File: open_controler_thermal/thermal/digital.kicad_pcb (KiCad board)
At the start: 2 copper layers, 56 x 85 mm, 6 parts, among them J1 d_o_01x10, J2 d_i_01x10, J3 Conn_02x20_Odd_Even, J4 Conn_01x02

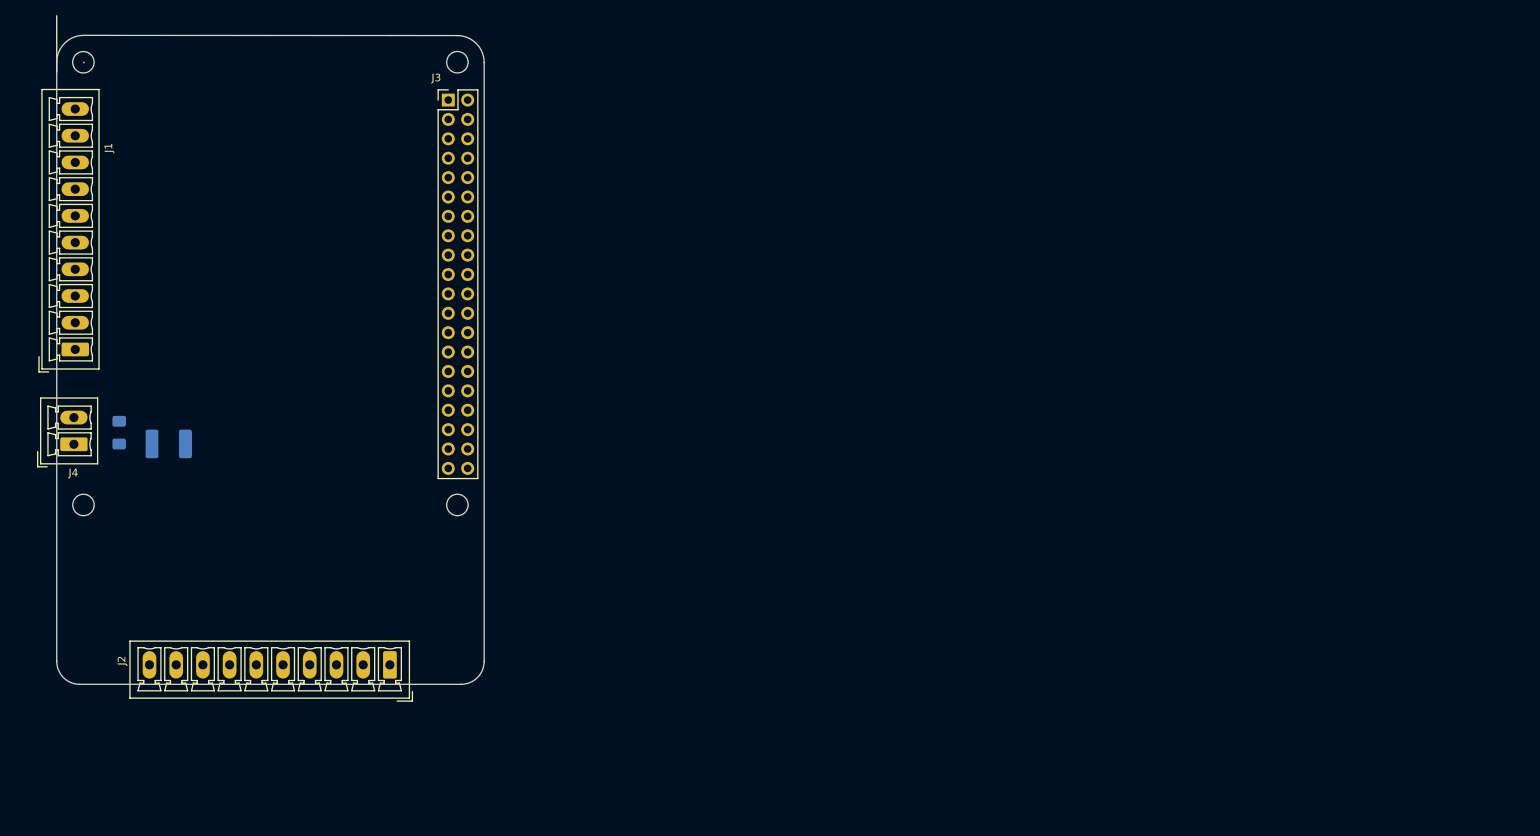
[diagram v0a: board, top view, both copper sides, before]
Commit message: trabajando en openControllerDigital
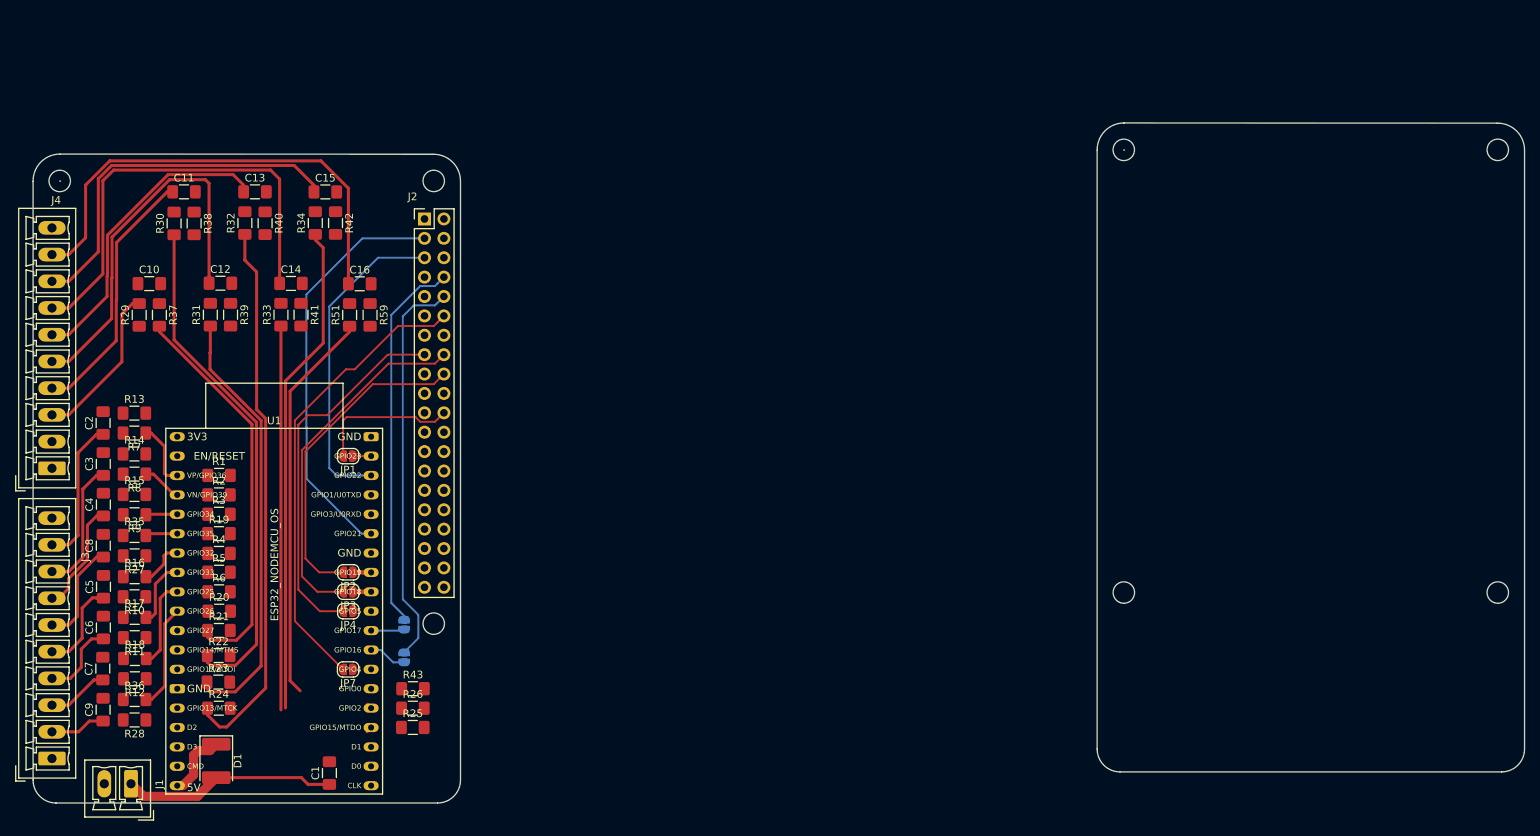
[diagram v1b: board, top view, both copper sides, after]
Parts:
- removed the J1 at (75.7, 82.8)
- added C1: 10nF, Capacitor_SMD:C_1206_3216Metric_Pad1.42x1.75mm_HandSolder, F.Cu at (109.0, 138.3)
- added C10: 10nF, Capacitor_SMD:C_1206_3216Metric_Pad1.42x1.75mm_HandSolder, F.Cu at (85.4, 74.2)
- added C11: 10nF, Capacitor_SMD:C_1206_3216Metric_Pad1.42x1.75mm_HandSolder, F.Cu at (90.0, 62.2)
- added C12: 10nF, Capacitor_SMD:C_1206_3216Metric_Pad1.42x1.75mm_HandSolder, F.Cu at (94.7, 74.1)
- added C13: 10nF, Capacitor_SMD:C_1206_3216Metric_Pad1.42x1.75mm_HandSolder, F.Cu at (99.2, 62.2)
- added C14: 10nF, Capacitor_SMD:C_1206_3216Metric_Pad1.42x1.75mm_HandSolder, F.Cu at (104.0, 74.2)
- added C15: 10nF, Capacitor_SMD:C_1206_3216Metric_Pad1.42x1.75mm_HandSolder, F.Cu at (108.5, 62.2)
- added C16: 10nF, Capacitor_SMD:C_1206_3216Metric_Pad1.42x1.75mm_HandSolder, F.Cu at (113.0, 74.2)
- added C2: 10nF, Capacitor_SMD:C_1206_3216Metric_Pad1.42x1.75mm_HandSolder, F.Cu at (79.3, 92.5)
- added C3: 10nF, Capacitor_SMD:C_1206_3216Metric_Pad1.42x1.75mm_HandSolder, F.Cu at (79.4, 97.8)
- added C4: 10nF, Capacitor_SMD:C_1206_3216Metric_Pad1.42x1.75mm_HandSolder, F.Cu at (79.4, 103.2)
- added C5: 10nF, Capacitor_SMD:C_1206_3216Metric_Pad1.42x1.75mm_HandSolder, F.Cu at (79.4, 113.9)
- added C6: 10nF, Capacitor_SMD:C_1206_3216Metric_Pad1.42x1.75mm_HandSolder, F.Cu at (79.4, 119.3)
- added C8: 10nF, Capacitor_SMD:C_1206_3216Metric_Pad1.42x1.75mm_HandSolder, F.Cu at (79.4, 108.5)
- added C9: 10nF, Capacitor_SMD:C_1206_3216Metric_Pad1.42x1.75mm_HandSolder, F.Cu at (79.3, 130.0)
- added J4: e_i_01x10, Connector_Phoenix_MC:PhoenixContact_MCV_1,5_10-G-3.5_1x10_P3.50mm_Vertical, F.Cu at (72.7, 98.4)
- added JP1: 23, Jumper:SolderJumper-2_P1.3mm_Open_RoundedPad1.0x1.5mm, F.Cu at (111.5, 96.8)
- added JP2: 19, Jumper:SolderJumper-2_P1.3mm_Open_RoundedPad1.0x1.5mm, F.Cu at (111.5, 112.0)
- added JP3: 18, Jumper:SolderJumper-2_P1.3mm_Open_RoundedPad1.0x1.5mm, F.Cu at (111.5, 114.6)
- added JP4: 05, Jumper:SolderJumper-2_P1.3mm_Open_RoundedPad1.0x1.5mm, F.Cu at (111.5, 117.1)
- added JP5: tx, Jumper:SolderJumper-2_P1.3mm_Open_RoundedPad1.0x1.5mm, B.Cu at (118.8, 118.9)
- added JP6: rx, Jumper:SolderJumper-2_P1.3mm_Open_RoundedPad1.0x1.5mm, B.Cu at (118.8, 123.2)
- added JP7: 04, Jumper:SolderJumper-2_P1.3mm_Open_RoundedPad1.0x1.5mm, F.Cu at (111.5, 124.8)
- added R1: 4k7, Resistor_SMD:R_1206_3216Metric_Pad1.42x1.75mm_HandSolder, F.Cu at (94.5, 99.3)
- added R10: 10k, Resistor_SMD:R_1206_3216Metric_Pad1.42x1.75mm_HandSolder, F.Cu at (83.5, 115.2)
- added R11: 10k, Resistor_SMD:R_1206_3216Metric_Pad1.42x1.75mm_HandSolder, F.Cu at (83.5, 120.6)
- added R12: 10k, Resistor_SMD:R_1206_3216Metric_Pad1.42x1.75mm_HandSolder, F.Cu at (83.5, 126.0)
- added R13: 10k, Resistor_SMD:R_1206_3216Metric_Pad1.42x1.75mm_HandSolder, F.Cu at (83.5, 91.2)
- added R14: 10k, Resistor_SMD:R_1206_3216Metric_Pad1.42x1.75mm_HandSolder, F.Cu at (83.5, 96.5)
- added R15: 10k, Resistor_SMD:R_1206_3216Metric_Pad1.42x1.75mm_HandSolder, F.Cu at (83.5, 101.8)
- added R16: 10k, Resistor_SMD:R_1206_3216Metric_Pad1.42x1.75mm_HandSolder, F.Cu at (83.5, 112.6)
- added R17: 10k, Resistor_SMD:R_1206_3216Metric_Pad1.42x1.75mm_HandSolder, F.Cu at (83.5, 117.9)
- added R18: 10k, Resistor_SMD:R_1206_3216Metric_Pad1.42x1.75mm_HandSolder, F.Cu at (83.5, 123.3)
- added R19: 4k7, Resistor_SMD:R_1206_3216Metric_Pad1.42x1.75mm_HandSolder, F.Cu at (94.5, 107.0)
- added R2: 4k7, Resistor_SMD:R_1206_3216Metric_Pad1.42x1.75mm_HandSolder, F.Cu at (94.5, 101.9)
- added R20: 4k7, Resistor_SMD:R_1206_3216Metric_Pad1.42x1.75mm_HandSolder, F.Cu at (94.6, 117.1)
- added R21: 4k7, Resistor_SMD:R_1206_3216Metric_Pad1.42x1.75mm_HandSolder, F.Cu at (94.5, 119.6)
- added R22: 4k7, Resistor_SMD:R_1206_3216Metric_Pad1.42x1.75mm_HandSolder, F.Cu at (94.5, 122.9)
- added R23: 4k7, Resistor_SMD:R_1206_3216Metric_Pad1.42x1.75mm_HandSolder, F.Cu at (94.5, 126.4)
- added R24: 4k7, Resistor_SMD:R_1206_3216Metric_Pad1.42x1.75mm_HandSolder, F.Cu at (94.5, 129.8)
- added R25: 4k7, Resistor_SMD:R_1206_3216Metric_Pad1.42x1.75mm_HandSolder, F.Cu at (119.9, 132.3)
- added R26: 4k7, Resistor_SMD:R_1206_3216Metric_Pad1.42x1.75mm_HandSolder, F.Cu at (119.9, 129.8)
- added R27: 10k, Resistor_SMD:R_1206_3216Metric_Pad1.42x1.75mm_HandSolder, F.Cu at (83.5, 109.9)
- added R28: 10k, Resistor_SMD:R_1206_3216Metric_Pad1.42x1.75mm_HandSolder, F.Cu at (83.5, 131.4)
- added R29: 10k, Resistor_SMD:R_1206_3216Metric_Pad1.42x1.75mm_HandSolder, F.Cu at (84.1, 78.3)
- added R3: 4k7, Resistor_SMD:R_1206_3216Metric_Pad1.42x1.75mm_HandSolder, F.Cu at (94.5, 104.4)
- added R30: 10k, Resistor_SMD:R_1206_3216Metric_Pad1.42x1.75mm_HandSolder, F.Cu at (88.7, 66.3)
- added R31: 10k, Resistor_SMD:R_1206_3216Metric_Pad1.42x1.75mm_HandSolder, F.Cu at (93.4, 78.3)
- added R32: 10k, Resistor_SMD:R_1206_3216Metric_Pad1.42x1.75mm_HandSolder, F.Cu at (97.9, 66.3)
- added R33: 10k, Resistor_SMD:R_1206_3216Metric_Pad1.42x1.75mm_HandSolder, F.Cu at (102.7, 78.3)
- added R34: 10k, Resistor_SMD:R_1206_3216Metric_Pad1.42x1.75mm_HandSolder, F.Cu at (107.2, 66.3)
- added R35: 10k, Resistor_SMD:R_1206_3216Metric_Pad1.42x1.75mm_HandSolder, F.Cu at (83.5, 107.2)
- added R36: 10k, Resistor_SMD:R_1206_3216Metric_Pad1.42x1.75mm_HandSolder, F.Cu at (83.5, 128.7)
- added R37: 10k, Resistor_SMD:R_1206_3216Metric_Pad1.42x1.75mm_HandSolder, F.Cu at (86.7, 78.3)
- added R38: 10k, Resistor_SMD:R_1206_3216Metric_Pad1.42x1.75mm_HandSolder, F.Cu at (91.3, 66.3)
- added R39: 10k, Resistor_SMD:R_1206_3216Metric_Pad1.42x1.75mm_HandSolder, F.Cu at (96.0, 78.3)
- added R4: 4k7, Resistor_SMD:R_1206_3216Metric_Pad1.42x1.75mm_HandSolder, F.Cu at (94.5, 109.5)
- added R40: 10k, Resistor_SMD:R_1206_3216Metric_Pad1.42x1.75mm_HandSolder, F.Cu at (100.6, 66.3)
- added R41: 10k, Resistor_SMD:R_1206_3216Metric_Pad1.42x1.75mm_HandSolder, F.Cu at (105.3, 78.3)
- added R42: 10k, Resistor_SMD:R_1206_3216Metric_Pad1.42x1.75mm_HandSolder, F.Cu at (109.8, 66.3)
- added R43: 4k7, Resistor_SMD:R_1206_3216Metric_Pad1.42x1.75mm_HandSolder, F.Cu at (120.0, 127.3)
- added R5: 4k7, Resistor_SMD:R_1206_3216Metric_Pad1.42x1.75mm_HandSolder, F.Cu at (94.5, 112.0)
- added R51: 10k, Resistor_SMD:R_1206_3216Metric_Pad1.42x1.75mm_HandSolder, F.Cu at (111.7, 78.3)
- added R59: 10k, Resistor_SMD:R_1206_3216Metric_Pad1.42x1.75mm_HandSolder, F.Cu at (114.3, 78.3)
- added R6: 4k7, Resistor_SMD:R_1206_3216Metric_Pad1.42x1.75mm_HandSolder, F.Cu at (94.5, 114.6)
- added R7: 10k, Resistor_SMD:R_1206_3216Metric_Pad1.42x1.75mm_HandSolder, F.Cu at (83.5, 93.8)
- added R8: 10k, Resistor_SMD:R_1206_3216Metric_Pad1.42x1.75mm_HandSolder, F.Cu at (83.5, 99.2)
- added R9: 10k, Resistor_SMD:R_1206_3216Metric_Pad1.42x1.75mm_HandSolder, F.Cu at (83.5, 104.5)
- added U1: ESP32_NODEMCU_OS, Espressif:ESP32-DevKitC, F.Cu at (89.1, 94.3)
- C7: value 10 -> 10nF; moved to F.Cu
- D1: footprint Diode_SMD:D_2114_3652Metric -> Digital:D_2114_3652Metric; moved to F.Cu
- J2: value d_i_01x10 -> Conn_02x20_Odd_Even; footprint Connector_Phoenix_MC:PhoenixContact_MCV_1,5_10-G-3.5_1x10_P3.50mm_Vertical -> Connector_PinHeader_2.54mm:PinHeader_2x20_P2.54mm_Vertical
- J3: value Conn_02x20_Odd_Even -> a_i_01x10; footprint Connector_PinHeader_2.54mm:PinHeader_2x20_P2.54mm_Vertical -> Connector_Phoenix_MC:PhoenixContact_MCV_1,5_10-G-3.5_1x10_P3.50mm_Vertical
- moved J3 100.7 mm to (72.7, 136.4), turned to 90 degrees
- moved J2 58.6 mm to (121.5, 65.7), turned to 0 degrees
- moved J1 45.1 mm to (83.0, 139.7), turned to 180 degrees
- moved D1 42.0 mm to (94.2, 136.7), turned to 270 degrees
- moved C7 31.0 mm to (79.3, 124.6)
- renumbered J4 to J1
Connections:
- net di20 renamed Net-(J2-Pad1)
- net di32 renamed Net-(J2-Pad7)
- C7 pad 1: 5v -> jA25
- C7 pad 2: GND_1 -> GND
- J1 pad 2: GND_1 -> GND
- J2 pad 10: GND_1 -> RXD
- J2 pad 2: di21 -> 5v_1
- J2 pad 3: di22 -> SDA
- J2 pad 4: gi2 -> 5v_1
- J2 pad 5: di30 -> SCL
- J2 pad 6: di31 -> GND
- J2 pad 8: gi3 -> TXD
- J2 pad 9: 5v_1 -> GND
- J3 pad 1: Net-(J3-Pad1) -> GND
- J3 pad 10: Net-(J3-Pad10) -> 3v3
- J3 pad 2: 5v_1 -> jA26
- J3 pad 3: Net-(J3-Pad3) -> jA25
- J3 pad 4: 5v_1 -> jA33
- J3 pad 5: Net-(J3-Pad5) -> jA32
- J3 pad 6: GND_1 -> jA35
- J3 pad 7: Net-(J3-Pad7) -> jA34
- J3 pad 8: Net-(J3-Pad8) -> jA39
- J3 pad 9: GND_1 -> jA36
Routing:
- net D13: track 0.00 -> 71.8 mm
- net D14: track 0.00 -> 66.8 mm
- net D02: track 0.00 -> 65.2 mm
- net jD00: track 0.00 -> 62.0 mm
- net o04: track 0.00 -> 60.4 mm
- net jD15: track 0.00 -> 58.6 mm
- net D12: track 0.00 -> 56.9 mm
- net SDA: track 0.00 -> 54.1 mm
- net RXD: track 0.00 -> 52.1 mm
- net D27: track 0.00 -> 51.8 mm
- net D00: track 0.00 -> 51.5 mm
- net D15: track 0.00 -> 51.1 mm
- net jD12: track 0.00 -> 50.0 mm
- net TXD: track 0.00 -> 49.6 mm
- net o05: track 0.00 -> 49.0 mm
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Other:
- board size 56 x 85 mm -> 195.4 x 89.1 mm
